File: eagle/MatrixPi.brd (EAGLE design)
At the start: 85 x 56 mm, 17 parts, among them U2 28-SOIC

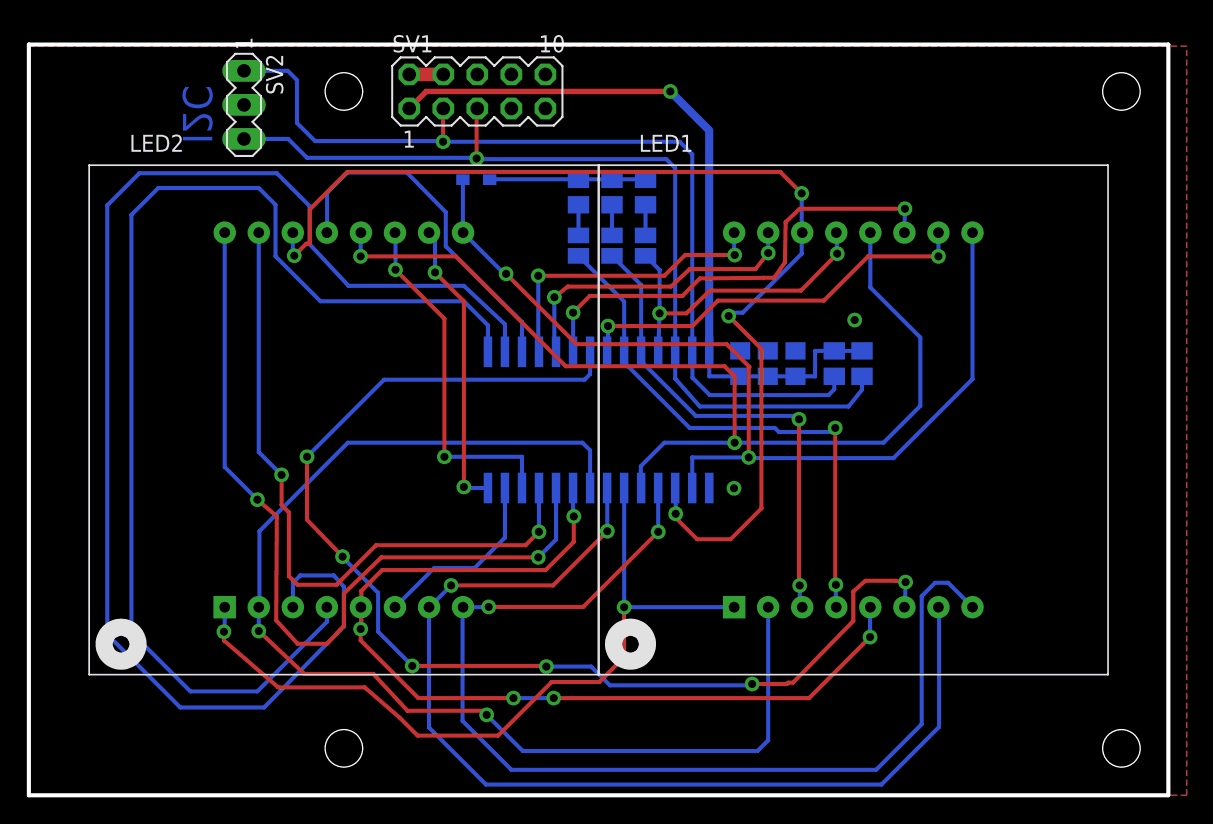
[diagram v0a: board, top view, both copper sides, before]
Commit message: brd
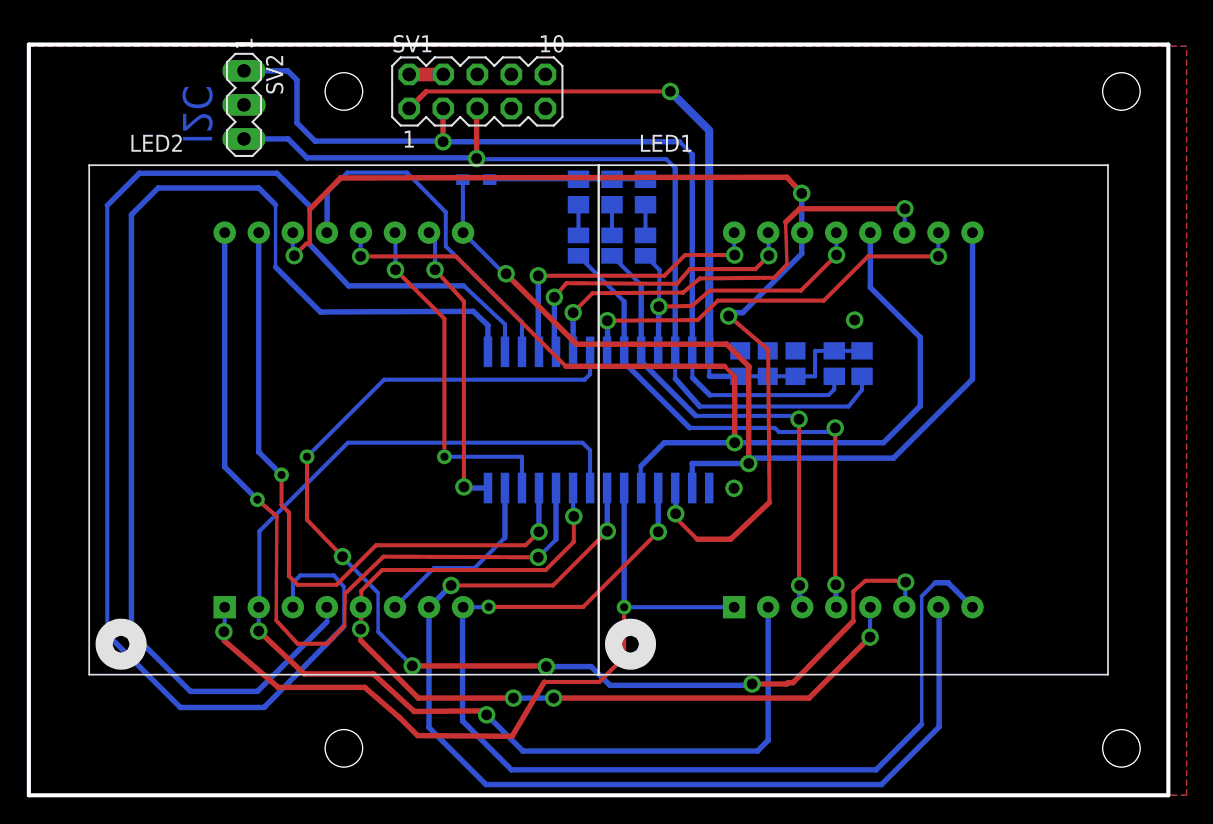
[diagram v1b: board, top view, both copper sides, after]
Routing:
- net N$4: track 58.3 -> 59.0 mm
